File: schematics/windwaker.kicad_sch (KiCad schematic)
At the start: 5 parts, among them SW1 SW_Push, U1 WEMOS_C3_mini, U2 TFT Display

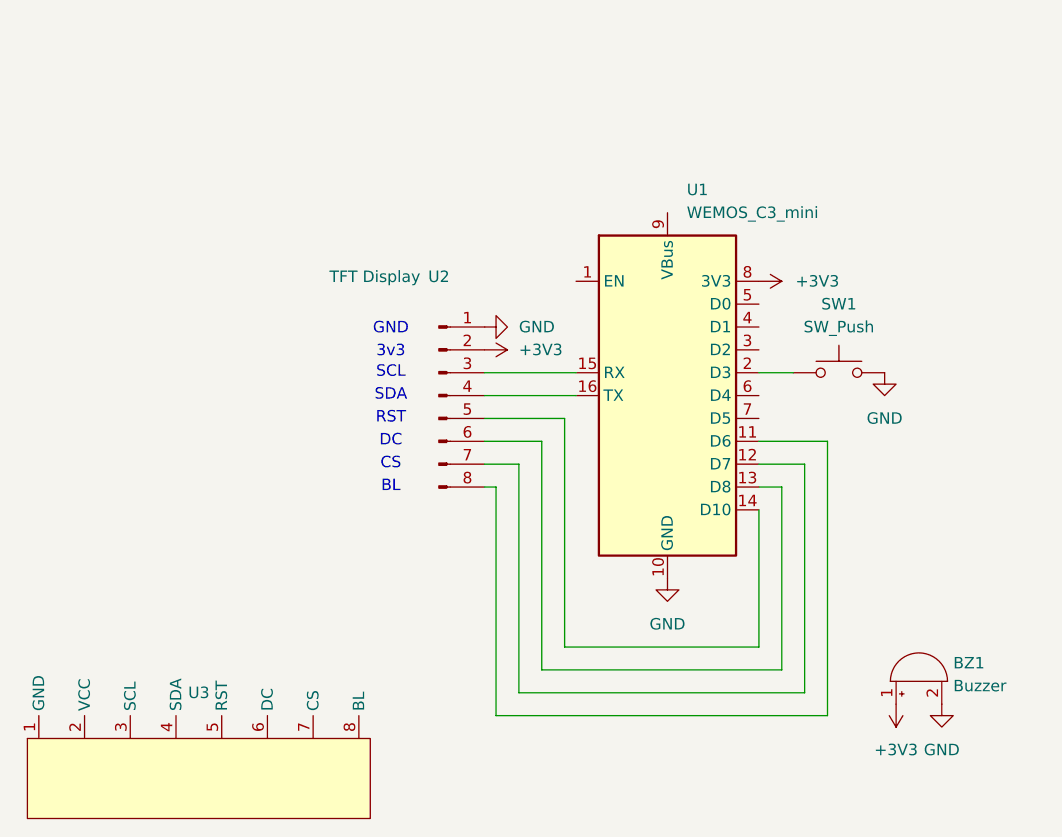
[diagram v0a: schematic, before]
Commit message: adding some 3d models and routing the pcb
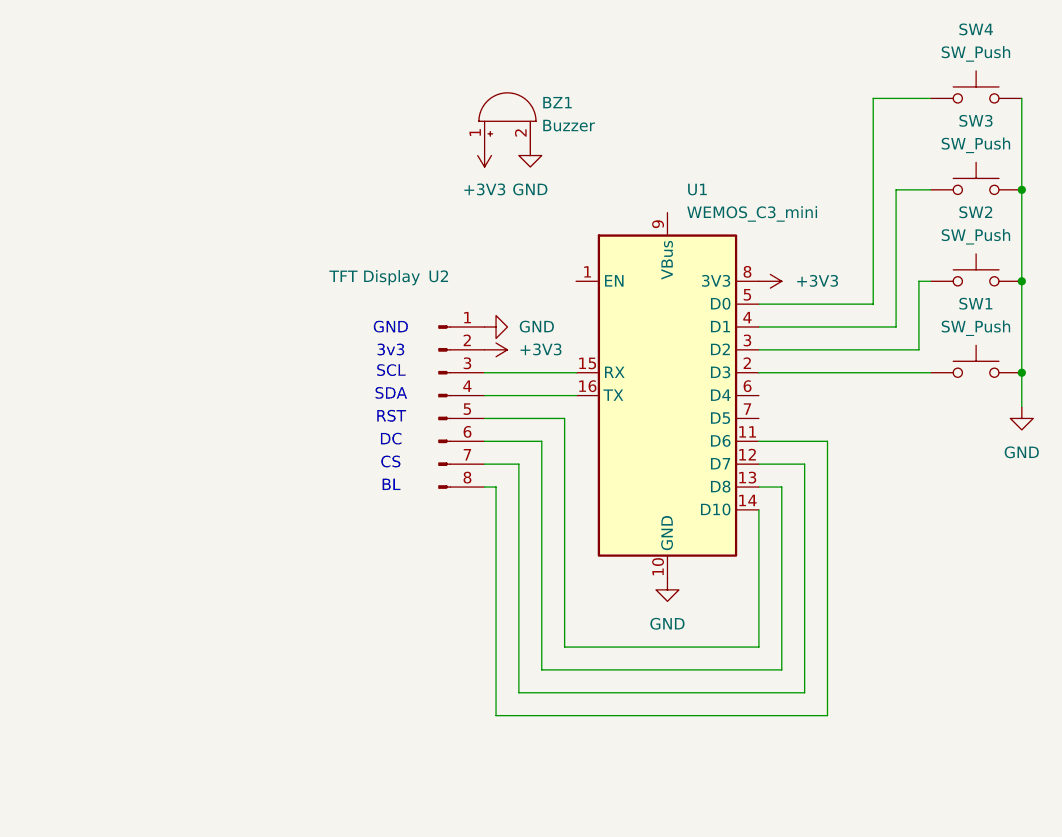
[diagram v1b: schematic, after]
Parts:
- removed U3: (no value), symbol my_custom_symbollib:TFT-display
- added SW2, SW3, SW4: SW_Push, Button_Switch_Keyboard:SW_Cherry_MX_1.00u_PCB, symbol Switch:SW_Push
- BZ1: footprint (none) -> my_custom_library:Buzzer_12x9.5RM7.6
- SW1: footprint (none) -> Button_Switch_Keyboard:SW_Cherry_MX_1.00u_PCB
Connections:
- net GND: now also SW2.2, SW3.2, SW4.2
- net at U1.3 (D2): now also SW2.1
- net at U1.4 (D1): now also SW3.1
- net at U1.5 (D0): now also SW4.1
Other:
- moved on the sheet: BZ1, SW1
